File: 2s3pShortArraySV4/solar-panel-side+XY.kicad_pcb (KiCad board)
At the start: 4 copper layers, 83 x 98 mm, 13 parts, among them J1 2053380005-CONNECTOR, U1 APDS9960_Breakout, U2 BNO080_Breakout, U3 MCP9808_Breakout

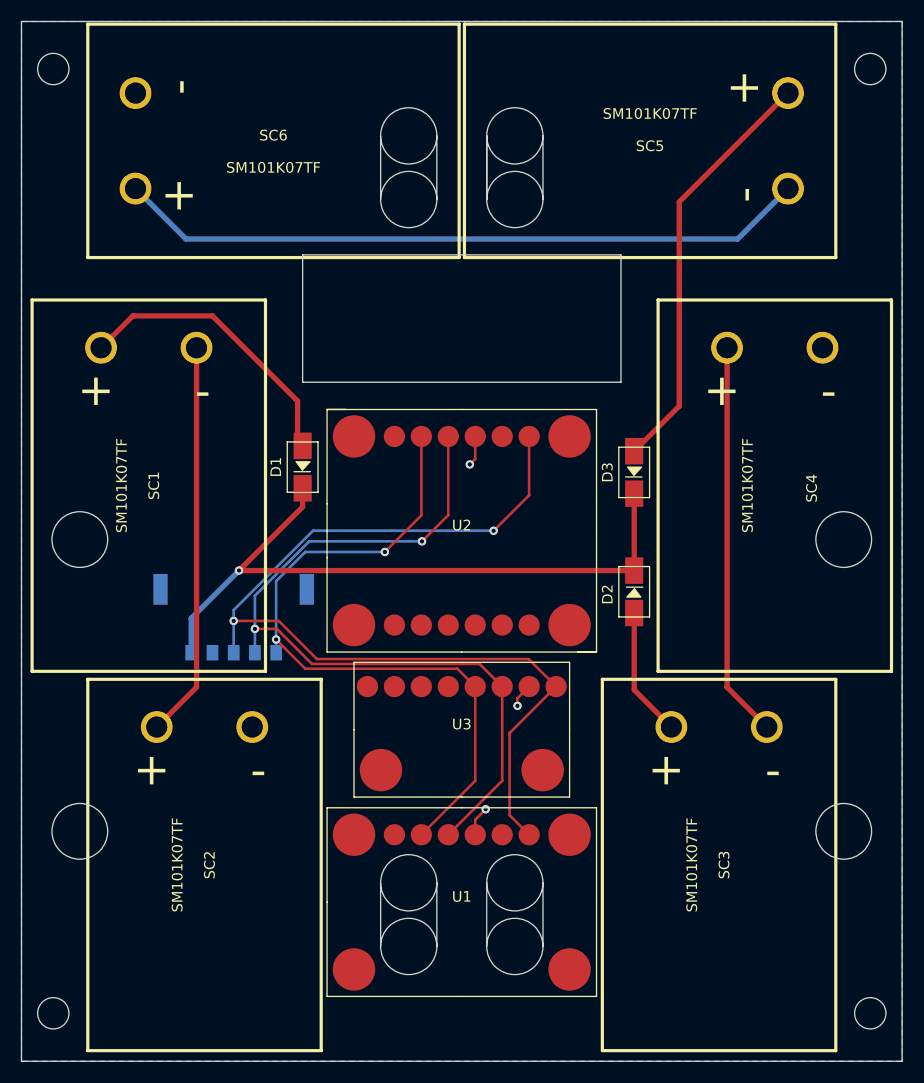
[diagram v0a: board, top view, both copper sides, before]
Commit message: Add files via upload
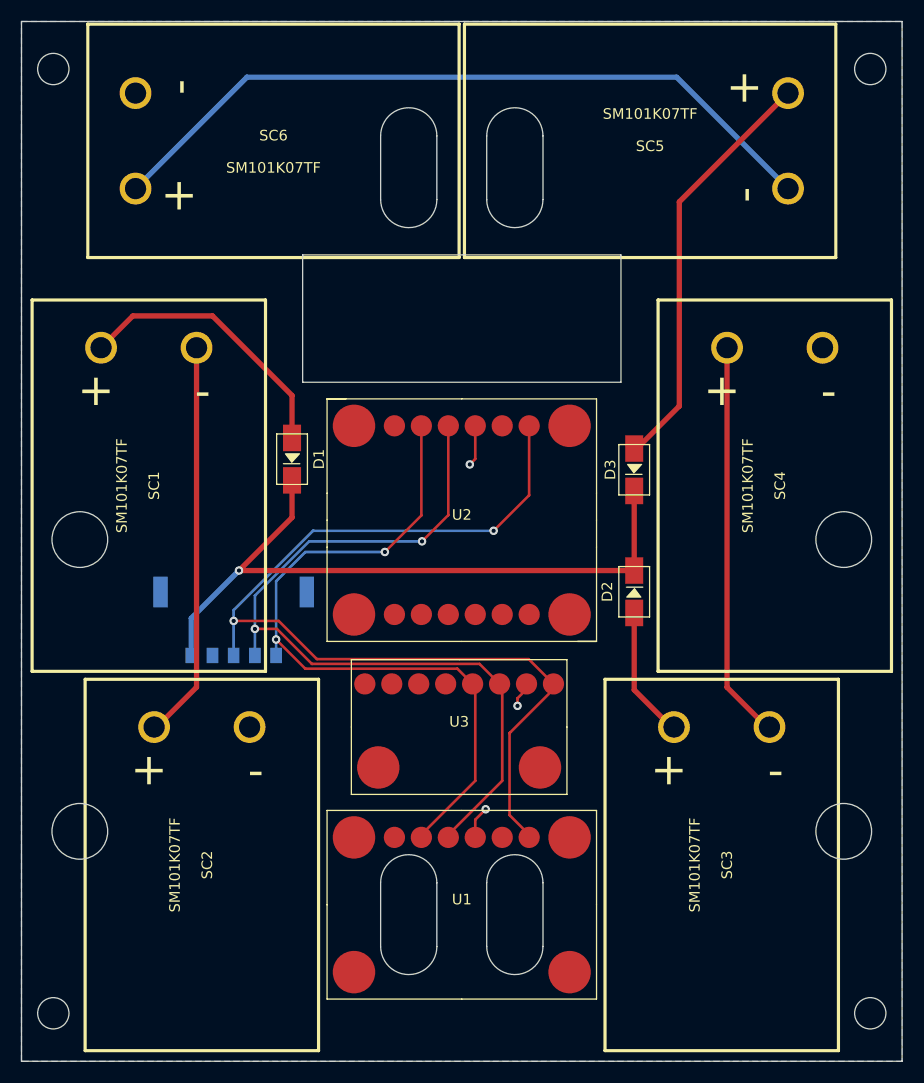
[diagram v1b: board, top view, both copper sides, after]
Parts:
- moved D1 1.25 mm to (125.5, 91.0)
- moved U2 1.00 mm to (141.5, 96.8)
- moved U3 0.35 mm to (141.2, 116.2)
- moved D3 0.25 mm to (157.8, 92.0)
- moved J1 0.25 mm to (116.0, 109.5)
- moved SC2 0.25 mm to (117.0, 129.2)
- moved SC3 0.25 mm to (166.0, 129.2)
- moved U1 0.25 mm to (141.5, 133.0)
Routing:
- net Net-(SC5-Pad2): track 65.4 -> 70.2 mm
- net Net-(D1-Pad2): track 28.3 -> 26.3 mm
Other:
- outline, holes or cut-outs redrawn
